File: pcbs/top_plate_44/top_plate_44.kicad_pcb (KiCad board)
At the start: 2 copper layers, 140.4 x 101.6 mm, 5 parts

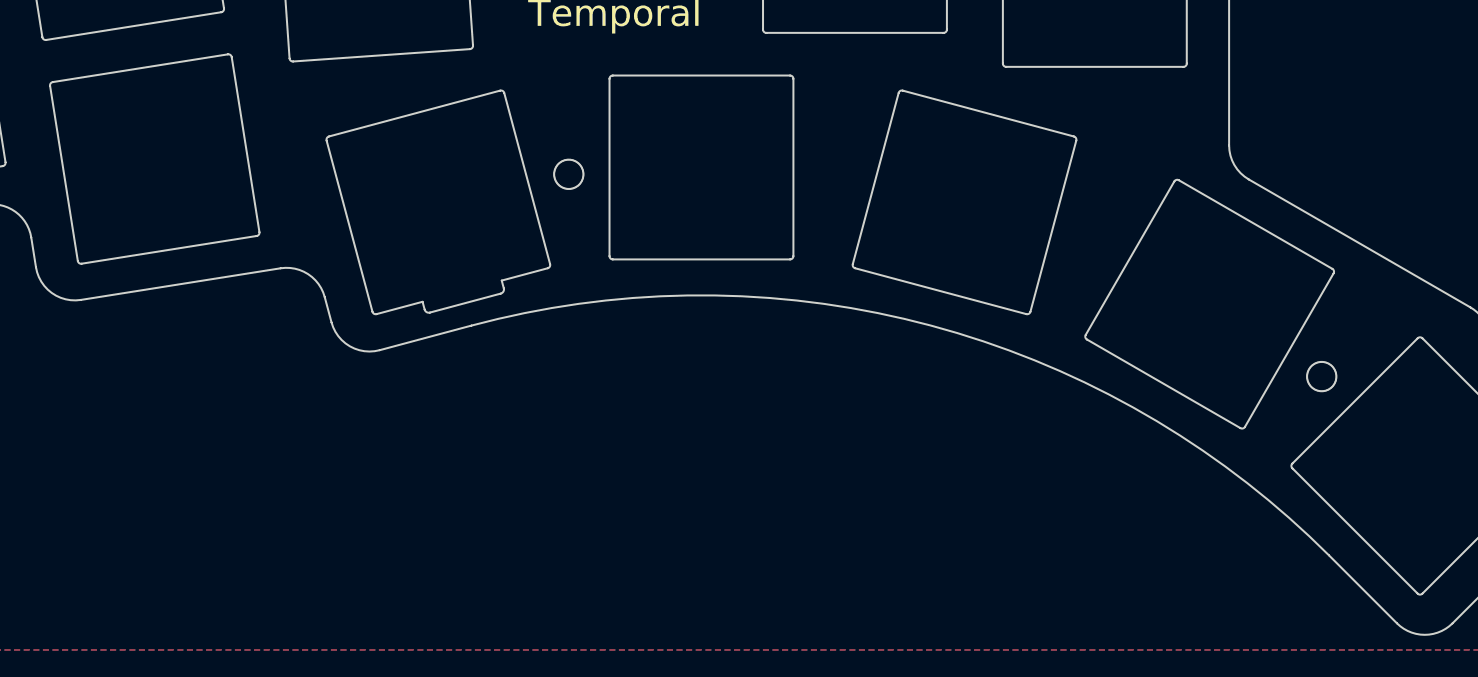
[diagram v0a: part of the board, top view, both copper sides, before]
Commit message: update gen files
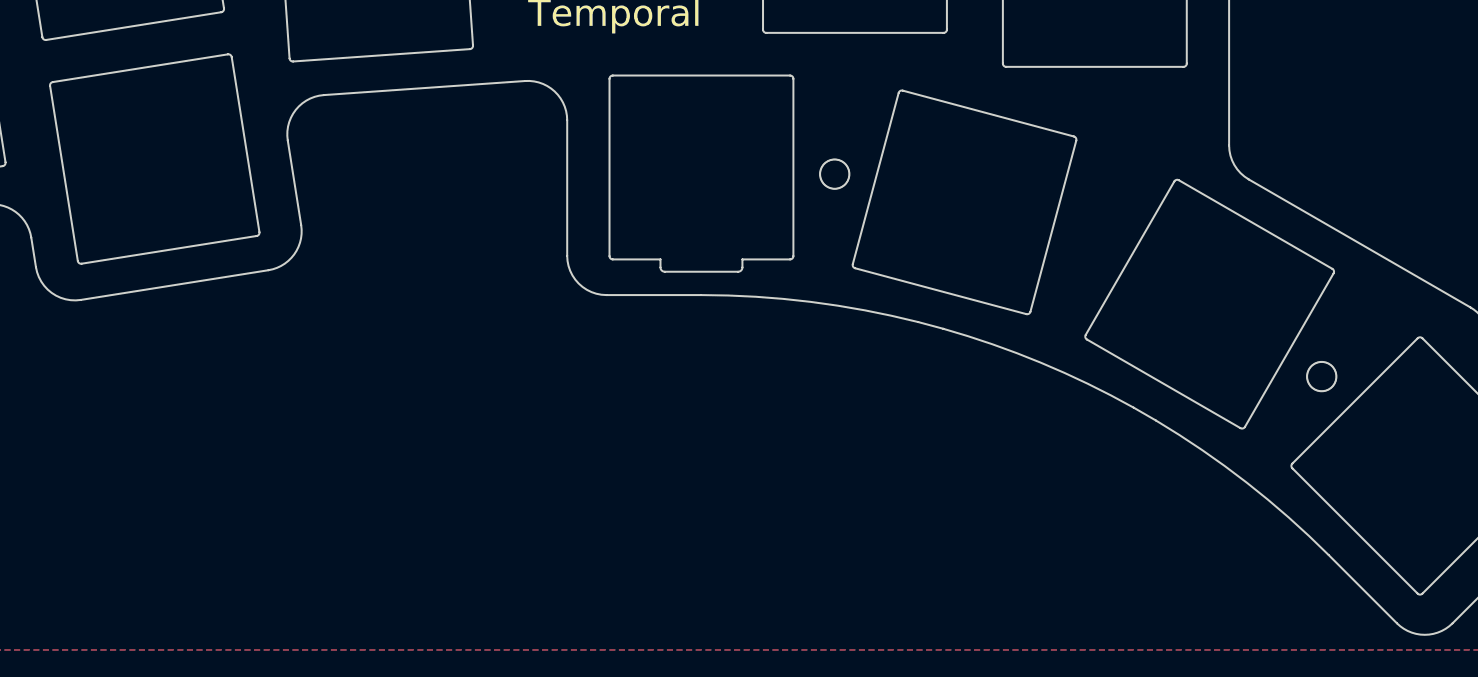
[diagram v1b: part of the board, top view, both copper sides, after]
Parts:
- moved MH4 20.0 mm to (117.4, 89.6), turned to 0 degrees
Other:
- outline, holes or cut-outs redrawn
